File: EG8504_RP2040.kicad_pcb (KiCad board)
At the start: 2 copper layers, 31.8 x 74.2 mm, 50 parts, among them J1 USB_C_Receptacle_USB2.0_16P, J2 522712079, J3 Conn_01x03_Socket, J4 Conn_01x14_Socket, J5 Conn_01x14_Socket, SW1 SW_Push, SW2 SW_Push, U1 RP2040, U2 W25Q16JVSS, U3 MIC5504-3.3YM5, U4 USBLC6-2SC6, U5 MC34063AD, Y1 ECS-3225MV-xxx-xx

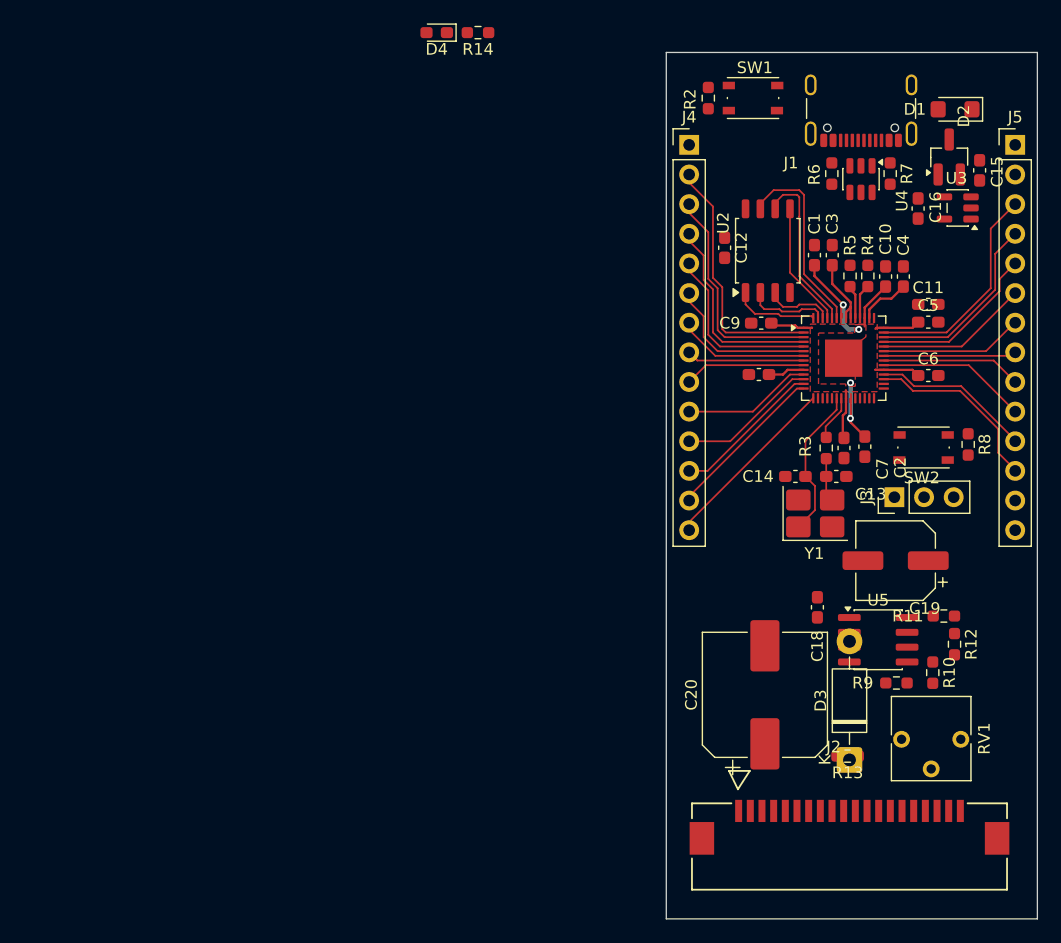
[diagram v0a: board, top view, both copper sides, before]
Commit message: sd入れたpsb
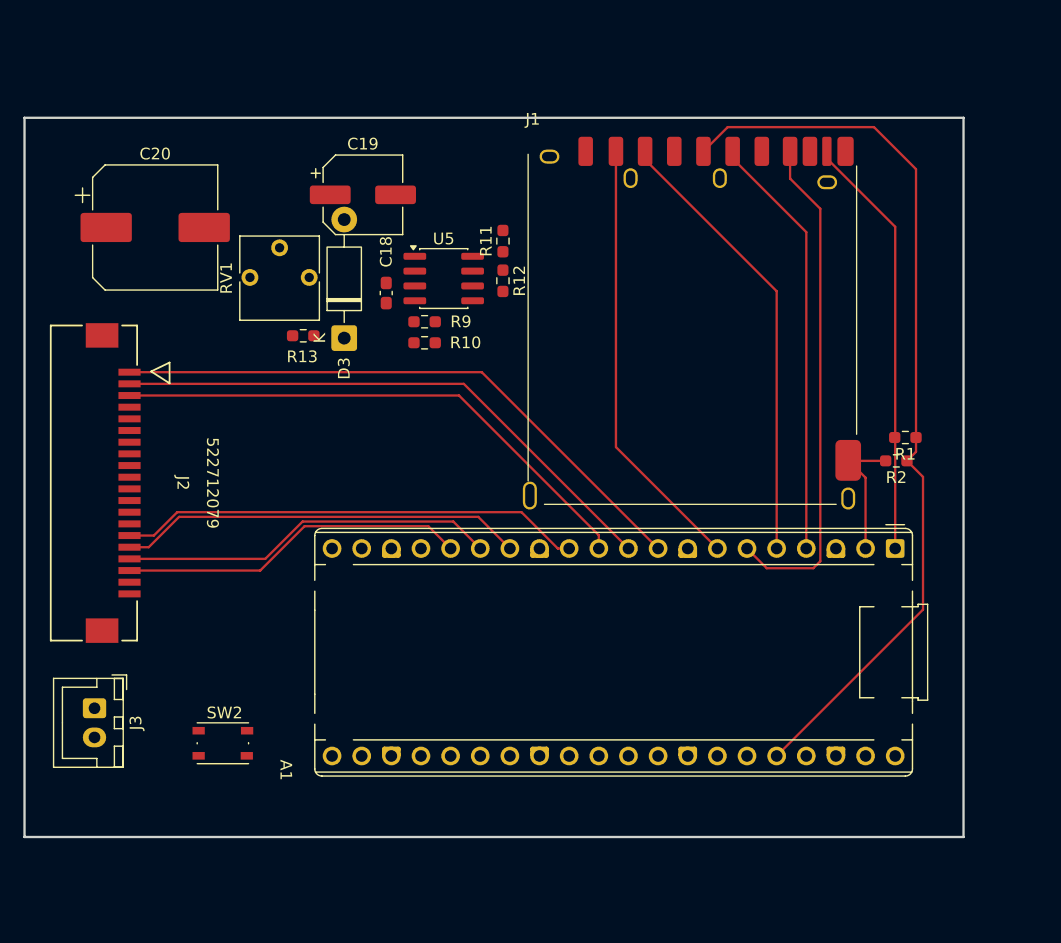
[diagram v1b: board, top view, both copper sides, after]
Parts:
- removed C1, C12, C2, C3, C4, C5, C6, C7, C8, C9: 100n, Capacitor_SMD:C_0603_1608Metric_Pad1.08x0.95mm_HandSolder
- removed C10, C11: 1u, Capacitor_SMD:C_0603_1608Metric_Pad1.08x0.95mm_HandSolder
- removed C13, C14: 22p, Capacitor_SMD:C_0603_1608Metric_Pad1.08x0.95mm_HandSolder
- removed C15, C16: 10u, Capacitor_SMD:C_0603_1608Metric_Pad1.08x0.95mm_HandSolder
- removed D1: SMF5V0A, Diode_SMD:D_SMF
- removed D2: CH213K, Package_TO_SOT_SMD:SOT-23_Handsoldering
- removed D4: LED_Small, LED_SMD:LED_0603_1608Metric_Pad1.05x0.95mm_HandSolder
- removed J4, J5: Conn_01x14_Socket, Connector_PinHeader_2.54mm:PinHeader_1x14_P2.54mm_Vertical
- removed R14, R3: 1k, Resistor_SMD:R_0603_1608Metric_Pad0.98x0.95mm_HandSolder
- removed R4, R5: 27, Resistor_SMD:R_0603_1608Metric_Pad0.98x0.95mm_HandSolder
- removed R6, R7: 5k1, Resistor_SMD:R_0603_1608Metric_Pad0.98x0.95mm_HandSolder
- removed R8: 10k, Resistor_SMD:R_0603_1608Metric_Pad0.98x0.95mm_HandSolder
- removed SW1: SW_Push, Button_Switch_SMD:SW_Push_1P1T_NO_Vertical_Wuerth_434133025816
- removed U1: RP2040, Package_DFN_QFN:QFN-56-1EP_7x7mm_P0.4mm_EP3.2x3.2mm
- removed U2: W25Q16JVSS, Package_SO:SOIC-8_5.3x5.3mm_P1.27mm
- removed U3: MIC5504-3.3YM5, Package_TO_SOT_SMD:SOT-23-5
- removed U4: USBLC6-2SC6, Package_TO_SOT_SMD:SOT-23-6
- removed Y1: ECS-3225MV-xxx-xx, Crystal:Crystal_SMD_3225-4Pin_3.2x2.5mm_HandSoldering
- added A1: RaspberryPi_Pico, Module:RaspberryPi_Pico_Common_THT, F.Cu at (129.4, 105.7)
- added R1: 10k, Resistor_SMD:R_0603_1608Metric_Pad0.98x0.95mm_HandSolder, F.Cu at (130.3, 96.2)
- J1: value USB_C_Receptacle_USB2.0_16P -> DM1B-DSF-PEJ; footprint Connector_USB:USB_C_Receptacle_GCT_USB4105-xx-A_16P_TopMnt_Horizontal -> MyLibrary:DM1B-DSF-PEJ
- J3: value Conn_01x03_Socket -> Conn_01x02_Socket; footprint Connector_PinHeader_2.54mm:PinHeader_1x03_P2.54mm_Vertical -> Connector_JST:JST_XH_B2B-XH-A_1x02_P2.50mm_Vertical
- R2: value 1k -> 10k
- moved J2 71.9 mm to (60.8, 100.1), turned to -90 degrees
- moved J3 70.9 mm to (60.8, 119.4), turned to -90 degrees
- moved C20 65.8 mm to (66.0, 78.2), turned to 0 degrees
- moved SW2 65.2 mm to (71.8, 122.4), turned to 0 degrees
- moved RV1 64.4 mm to (79.2, 82.5), turned to 90 degrees
- moved R13 58.9 mm to (78.7, 87.5), turned to 0 degrees
- moved D3 56.4 mm to (82.2, 87.7)
- moved C19 55.4 mm to (83.8, 75.4), turned to 0 degrees
- moved R10 51.9 mm to (89.1, 88.1), turned to 180 degrees
- moved R9 50.9 mm to (89.1, 86.3)
- moved R12 49.7 mm to (95.8, 82.8)
- moved R11 49.6 mm to (95.8, 79.4), turned to 90 degrees
- moved U5 48.4 mm to (90.7, 82.6)
- moved C18 45.7 mm to (85.8, 83.8), turned to -90 degrees
- moved R2 35.0 mm to (129.5, 98.2), turned to 180 degrees
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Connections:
- J2 pad 2: /GPIO14 -> /GPIO7
- J2 pad 3: /GPIO15 -> /GPIO8
- J3 pad 1: /SWD -> +5V
- R2 pad 1: Net-(R2-Pad1) -> +3.3V
- R2 pad 2: /QSPI_SS -> /GPIO1
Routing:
- net /DIN: track 0.00 -> 51.6 mm
- net +3.3V: track 29.7 -> 76.9 mm
- net /DAT0: track 0.00 -> 43.4 mm
- net /D4: track 0.00 -> 39.8 mm
- net /CMD: track 0.00 -> 38.7 mm
- net /GPIO7: track 10.4 -> 48.6 mm
- net /CD/DAT3: track 0.00 -> 37.6 mm
- net /CLK: track 0.00 -> 36.6 mm
- net /CD: track 0.00 -> 36.5 mm
- net /GPIO8: track 11.1 -> 46.3 mm
- net /D5: track 0.00 -> 34.8 mm
- net /D6: track 0.00 -> 32.3 mm
- net /D7: track 0.00 -> 29.9 mm
- net /GPIO0: track 21.5 -> 0.00 mm
- net +1V1: track 19.8 -> 0.00 mm, vias 4 -> 0
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- removed copper zone on F.Cu, net +1V1
- removed copper zone on F.Cu, net +3.3V
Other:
- board size 31.8 x 74.2 mm -> 80.5 x 61.6 mm
